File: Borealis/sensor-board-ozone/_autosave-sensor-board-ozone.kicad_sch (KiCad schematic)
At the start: 7 parts, among them J1 Conn_01x02_Pin (Solar panel c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, J2 Conn_01x03_Pin (data connecti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, J5 Conn_01x03_Pin (power connect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

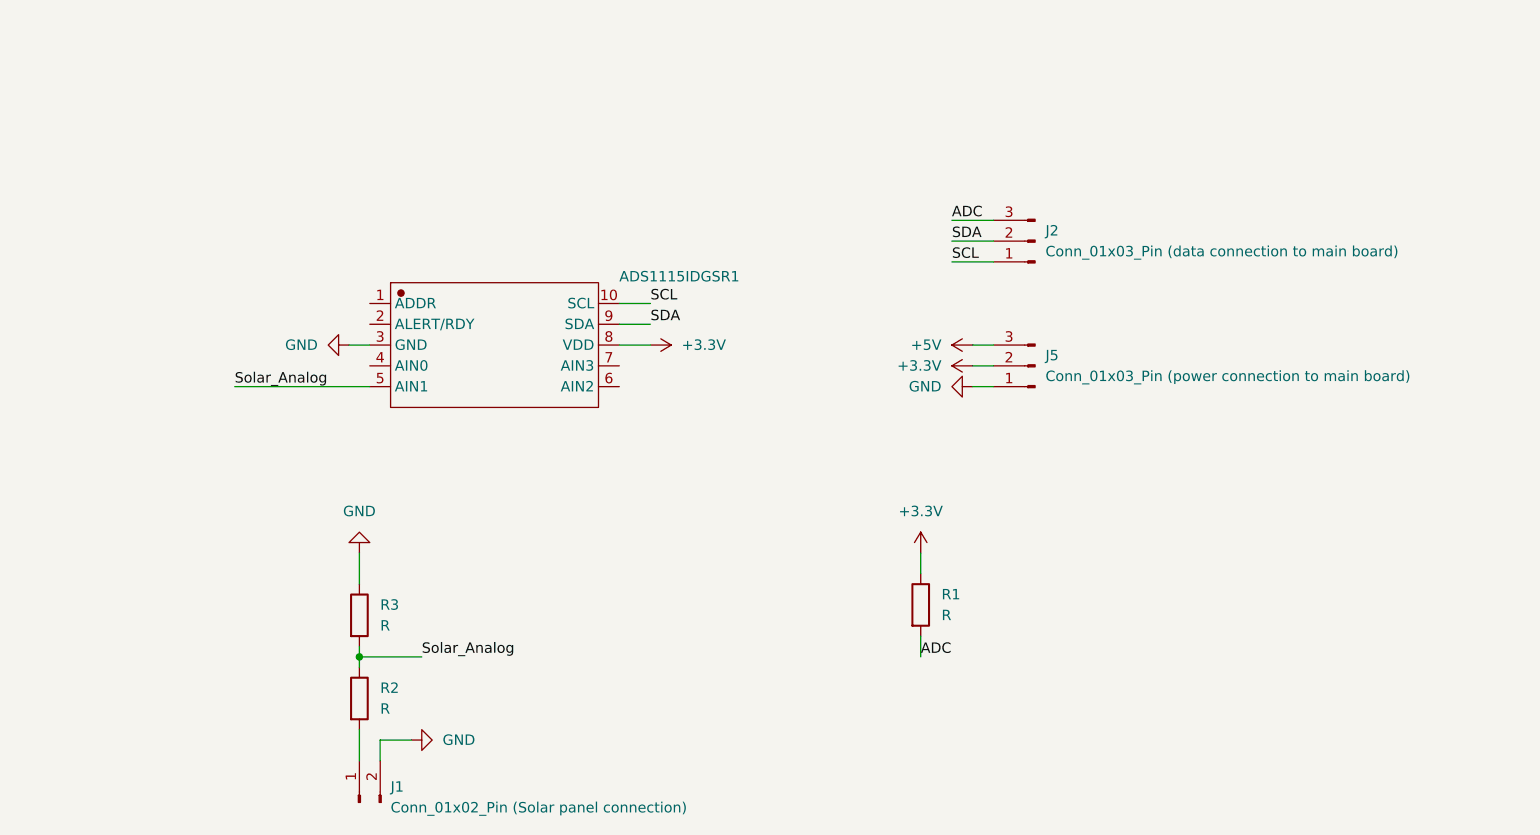
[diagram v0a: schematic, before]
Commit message: Updating changes
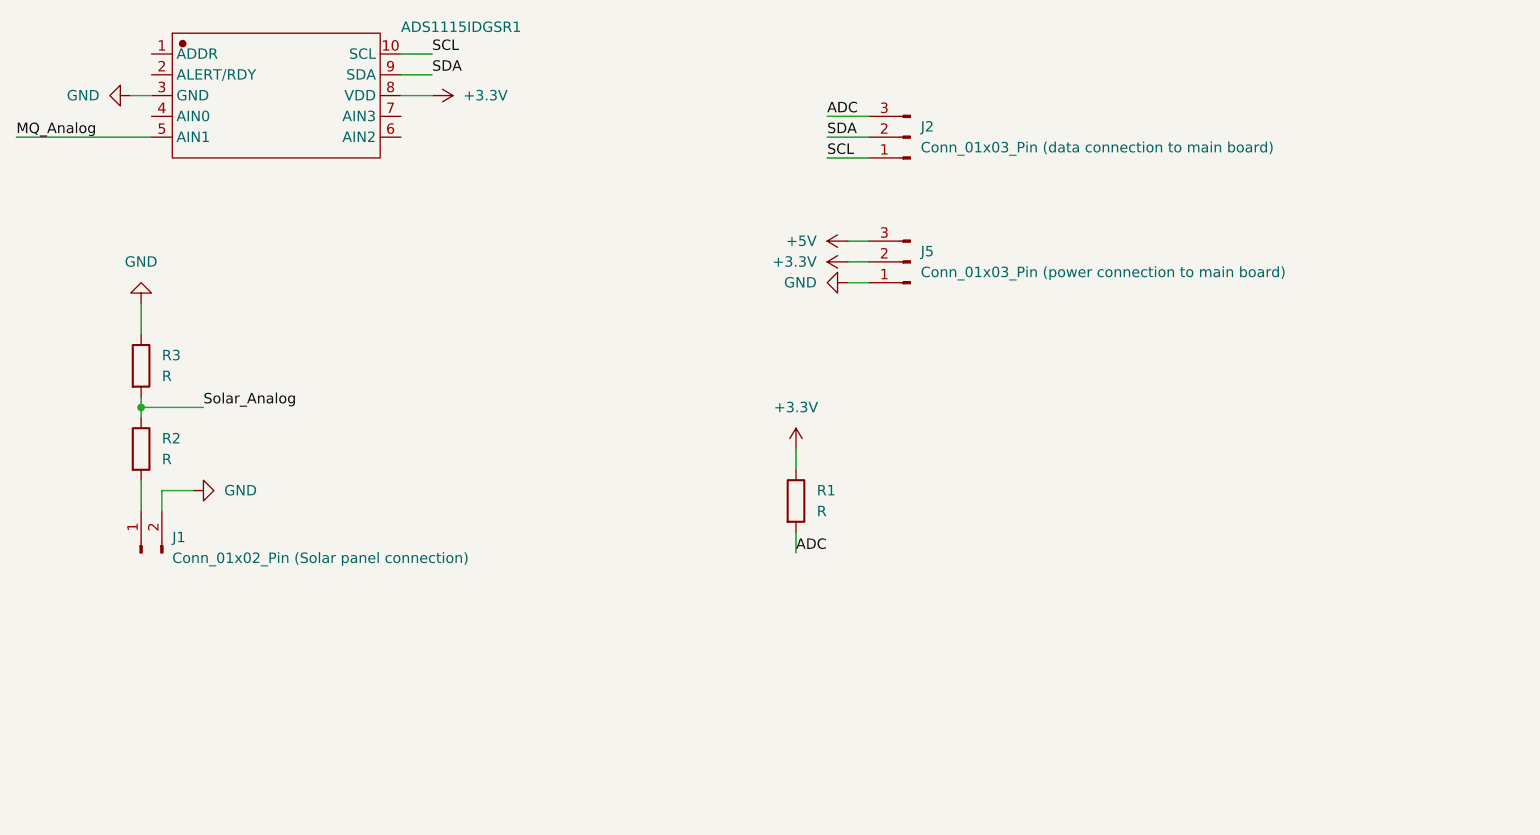
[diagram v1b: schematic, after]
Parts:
- J2, J5: footprint batteryholder:1x03 2.3 pitch -> (none)
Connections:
- net Solar_Analog: no longer ADS1115IDGSR1.5 (AIN1)
- new net MQ_Analog: ADS1115IDGSR1.5 (AIN1)
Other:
- moved on the sheet: ADS1115IDGSR1, J1, J2, J5, R1, R2, R3
